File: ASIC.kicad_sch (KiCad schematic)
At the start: 66 parts, among them U10 BM1370_mode1, U11 MCP1824T-1202E/OT, U12 MCP1824T-0802E, U2 SN74AVC4T774, U8 25MHz, U9 BM1370_mode1

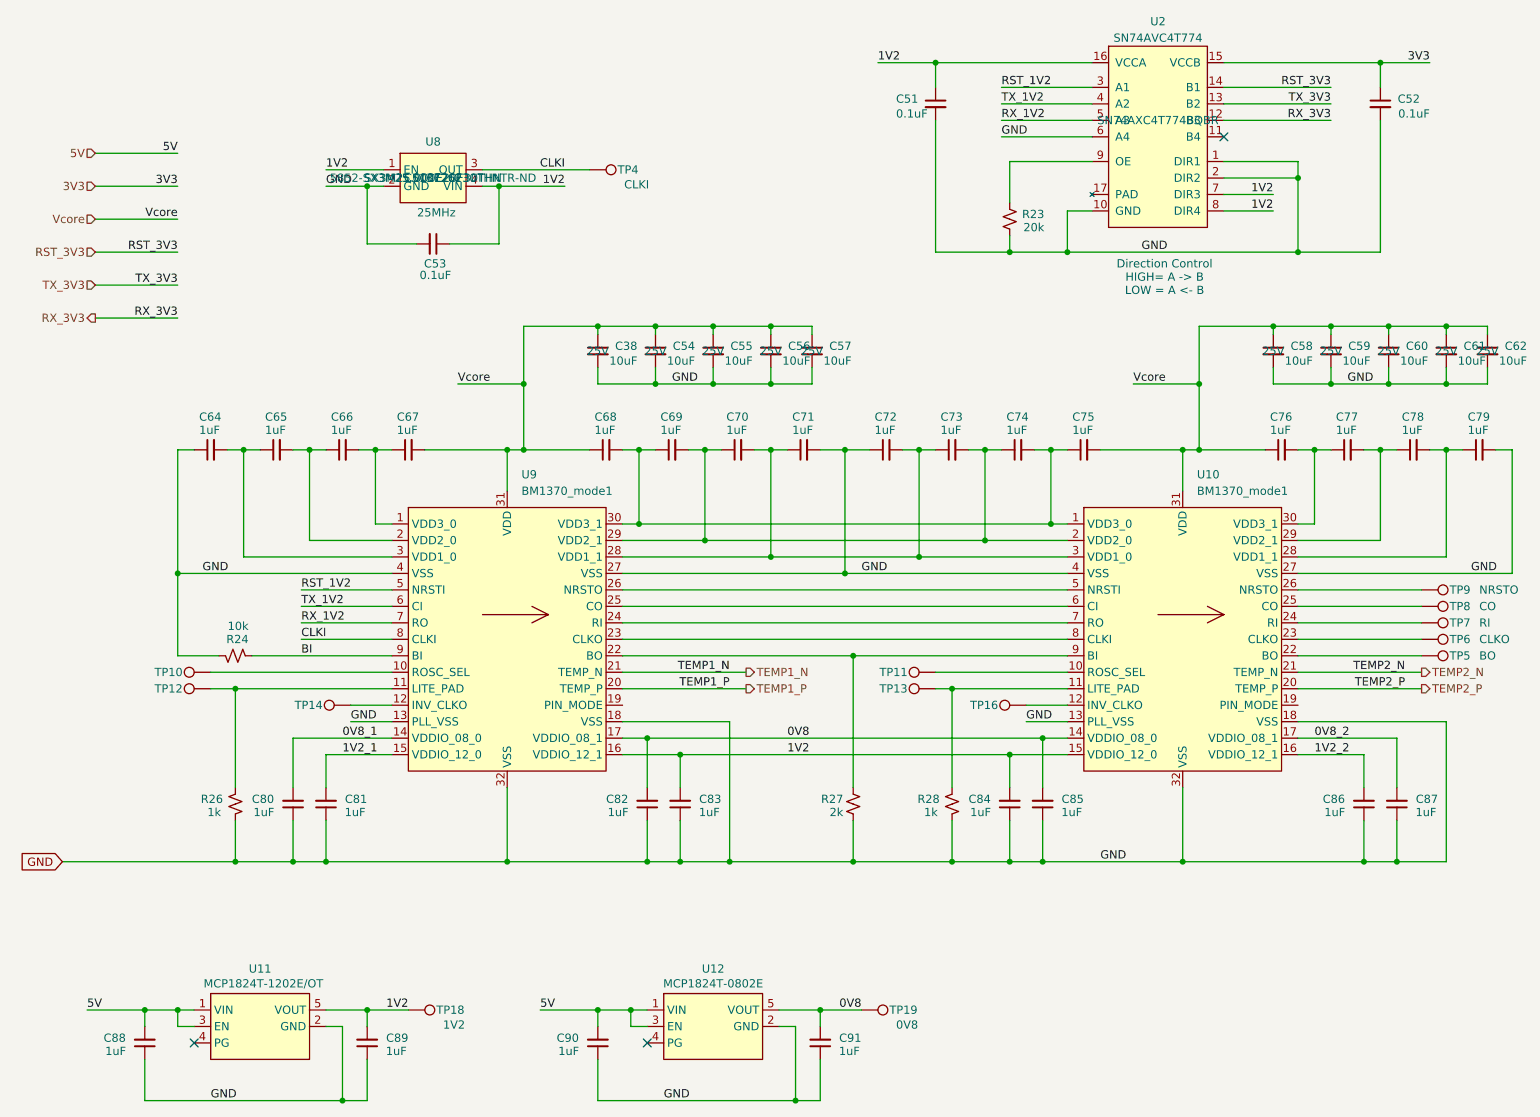
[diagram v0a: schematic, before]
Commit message: lots of routing
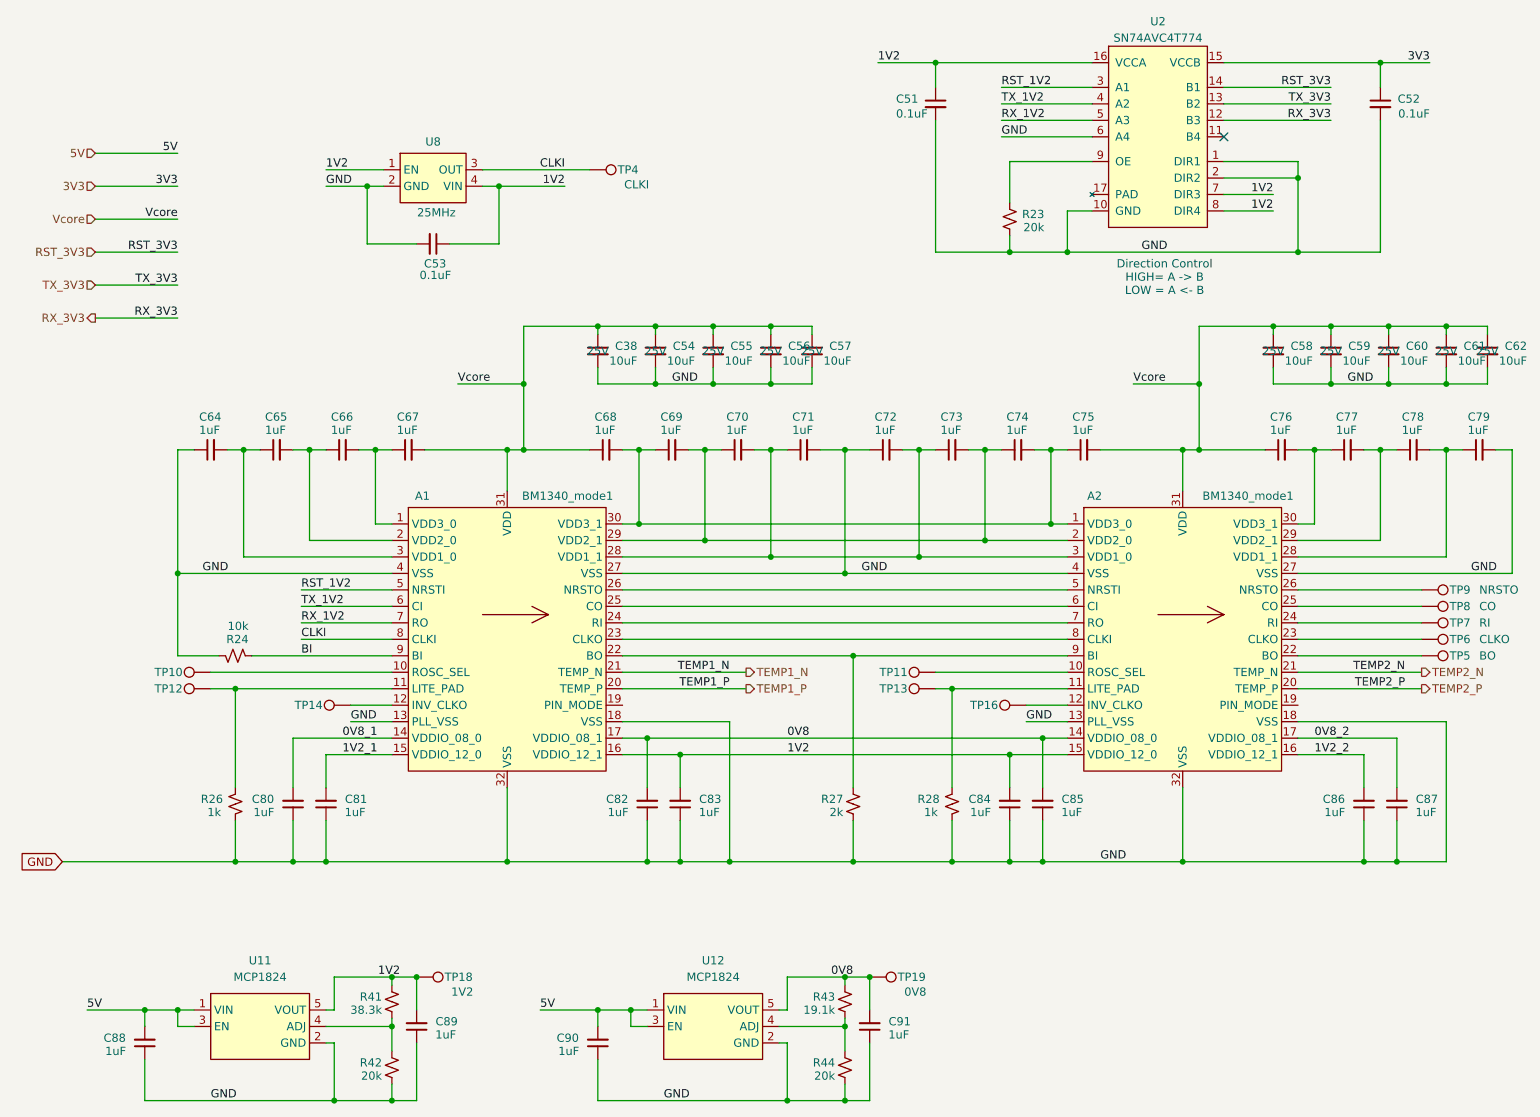
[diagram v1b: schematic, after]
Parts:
- removed U11: MCP1824T-1202E/OT, Package_TO_SOT_SMD:SOT-23-5, symbol bitaxe:MCP1824
- removed U12: MCP1824T-0802E, Package_TO_SOT_SMD:SOT-23-5, symbol bitaxe:MCP1824
- added R41: 38.3k, Resistor_SMD:R_0402_1005Metric, symbol Device:R_Small_US
- added R42, R44: 20k, Resistor_SMD:R_0402_1005Metric, symbol Device:R_Small_US
- added R43: 19.1k, Resistor_SMD:R_0402_1005Metric, symbol Device:R_Small_US
- added U11, U12: MCP1824, Package_TO_SOT_SMD:SOT-23-5, symbol bitaxe:MCP1824-ADJ
- A1: renamed from U9; value BM1370_mode1 -> BM1340_mode1; footprint bitaxe:BM1370 -> bitaxe:BM1340; symbol bitaxe:BM1370_mode1 -> bitaxe:BM1340_mode1
- A2: renamed from U10; value BM1370_mode1 -> BM1340_mode1; footprint bitaxe:BM1370 -> bitaxe:BM1340; symbol bitaxe:BM1370_mode1 -> bitaxe:BM1340_mode1
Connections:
- net 0V8: now also R43.2, U12.5 (VOUT)
- net 1V2: now also R41.2, U11.5 (VOUT)
- net 5V: now also U11.1 (VIN), U11.3 (EN), U12.1 (VIN), U12.3 (EN)
- net GND: now also R42.1, R44.1, U11.2 (GND), U12.2 (GND)
- new net: R41.1, R42.2, U11.4 (ADJ)
- new net: R43.1, R44.2, U12.4 (ADJ)
- no-connect marks 3 -> 1
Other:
- title: bitaxeGamma Turbo -> bitaxeNaja
- moved on the sheet: C89, C91, TP18, TP19
